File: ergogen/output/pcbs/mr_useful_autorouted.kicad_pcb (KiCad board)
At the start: 2 copper layers, 57 x 95 mm, 37 parts

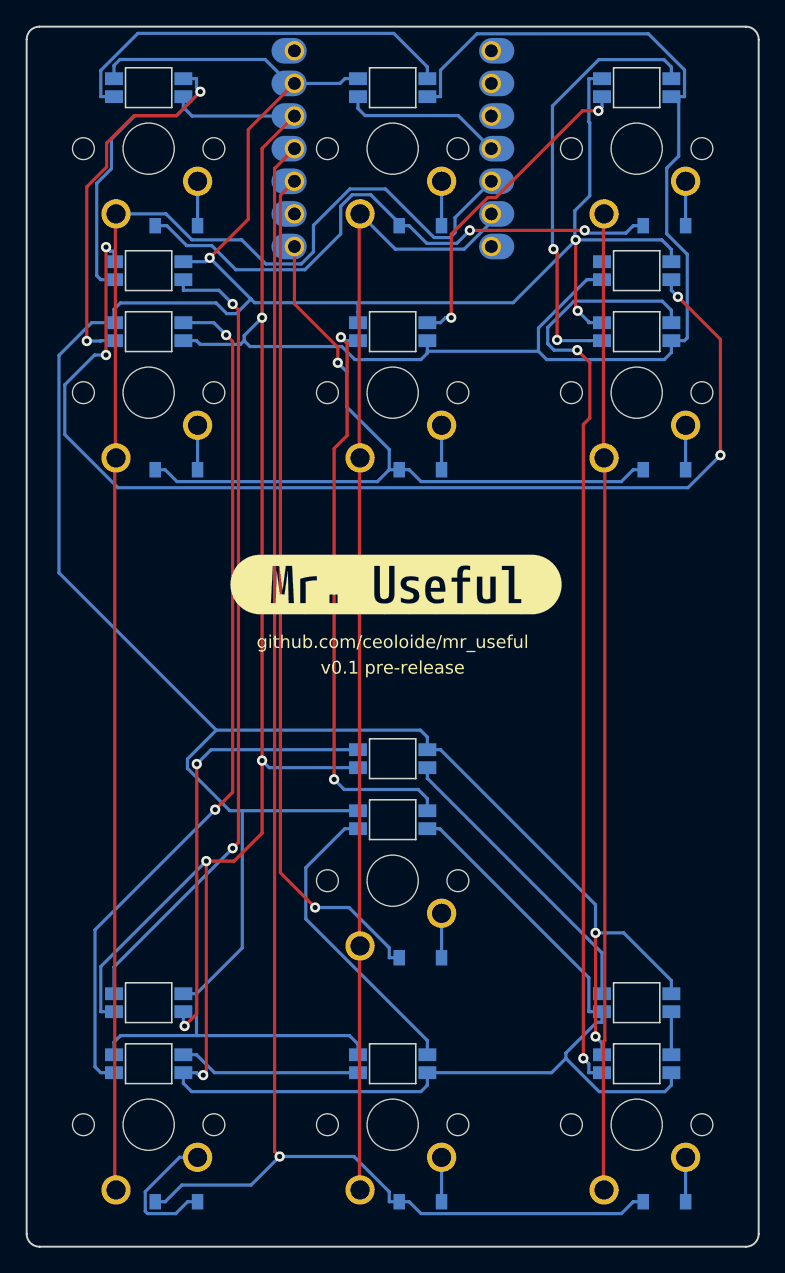
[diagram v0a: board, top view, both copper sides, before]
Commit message: Update assets
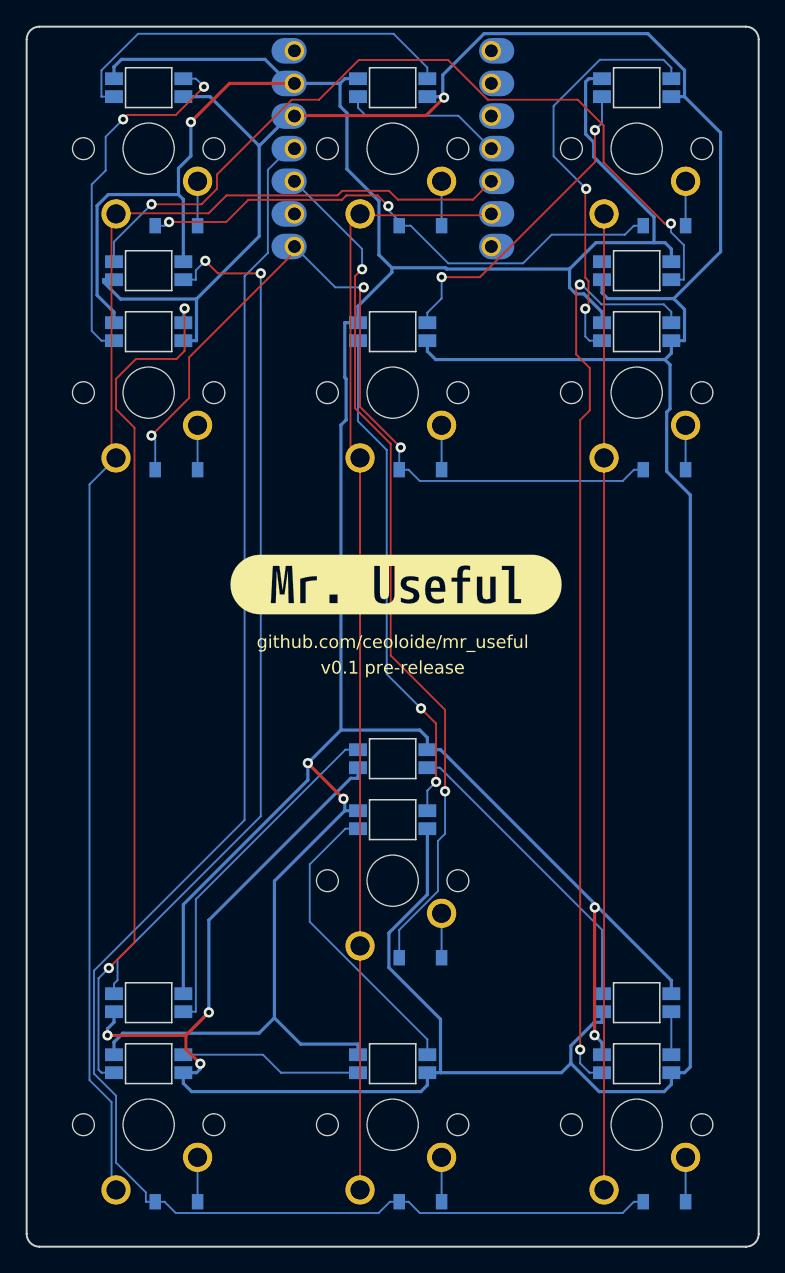
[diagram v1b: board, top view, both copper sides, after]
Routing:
- net ULED_4: track 87.1 -> 64.1 mm, vias 4 -> 2
- net R0: track 121.8 -> 130.6 mm, vias 1 -> 0
- net ULED_2: track 35.0 -> 27.2 mm, vias 2 -> 0
- net left_down: track 11.2 -> 3.46 mm
- net VCC: track 303.3 -> 296.1 mm
- net LED_6: track 45.3 -> 39.4 mm
- net C0: track 115.1 -> 109.3 mm
- net GND: track 272.2 -> 277.7 mm
- net ULED_3: track 63.0 -> 68.3 mm
- net R3: track 60.4 -> 64.6 mm, vias 1 -> 3
- net R4: track 45.6 -> 42.9 mm
- net C1: track 89.4 -> 87.3 mm
- net LED_8: track 33.8 -> 32.4 mm
- net LED_9: track 73.6 -> 72.4 mm
- net ULED_1: track 23.2 -> 23.8 mm
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
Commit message: Update assets
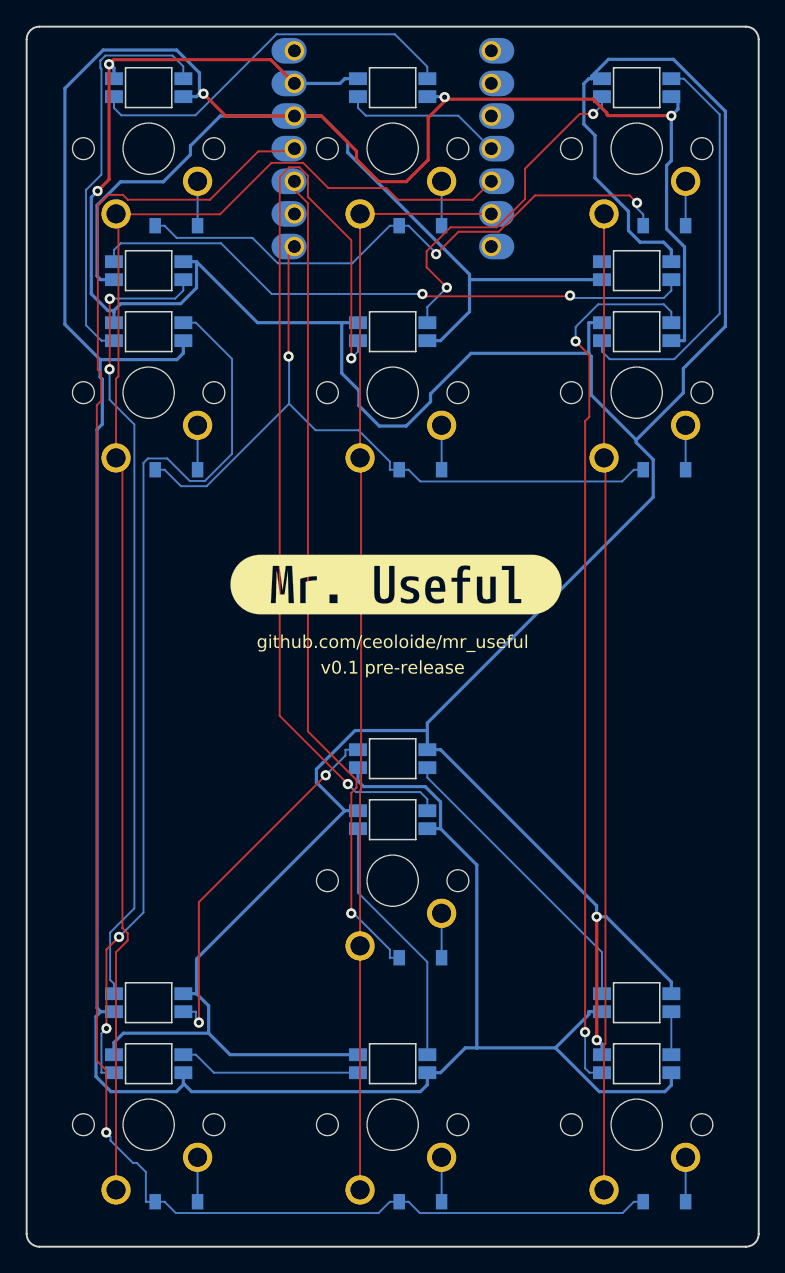
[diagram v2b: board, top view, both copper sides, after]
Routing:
- net LED_6: track 39.4 -> 77.0 mm
- net VCC: track 296.1 -> 318.8 mm, vias 4 -> 3
- net GND: track 277.7 -> 299.6 mm, vias 5 -> 4
- net ULED_4: track 64.1 -> 47.4 mm
- net R3: track 64.6 -> 57.3 mm, vias 3 -> 1
- net R0: track 130.6 -> 137.6 mm, vias 0 -> 1
- net ULED_3: track 68.3 -> 62.7 mm
- net LED_5: track 23.5 -> 19.8 mm
- net LED_9: track 72.4 -> 69.0 mm
- net LED_3: track 67.5 -> 70.8 mm
- net LED_2: track 28.8 -> 31.7 mm, vias 2 -> 0
- net R1: track 67.7 -> 65.1 mm, vias 2 -> 1
- net LED_7: track 25.0 -> 27.3 mm
- net R4: track 42.9 -> 45.0 mm
- net ULED_2: track 27.2 -> 28.9 mm, vias 0 -> 2
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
